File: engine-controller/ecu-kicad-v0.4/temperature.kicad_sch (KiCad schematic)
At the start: 70 parts, among them U31 AD8495, U32 TL431DBZ, U33 AD8495, U34 TL431DBZ, U35 AD8495, U36 AD8495, U37 TL431DBZ, U38 TL431DBZ, U39 AD8495, U40 TL431DBZ, U41 AD8495, U42 AD8495, U43 AD8495, U44 AD8495, U45 AD8495, U46 TL431DBZ, U47 TL431DBZ, U48 TL431DBZ, U49 TL431DBZ, U50 TL431DBZ

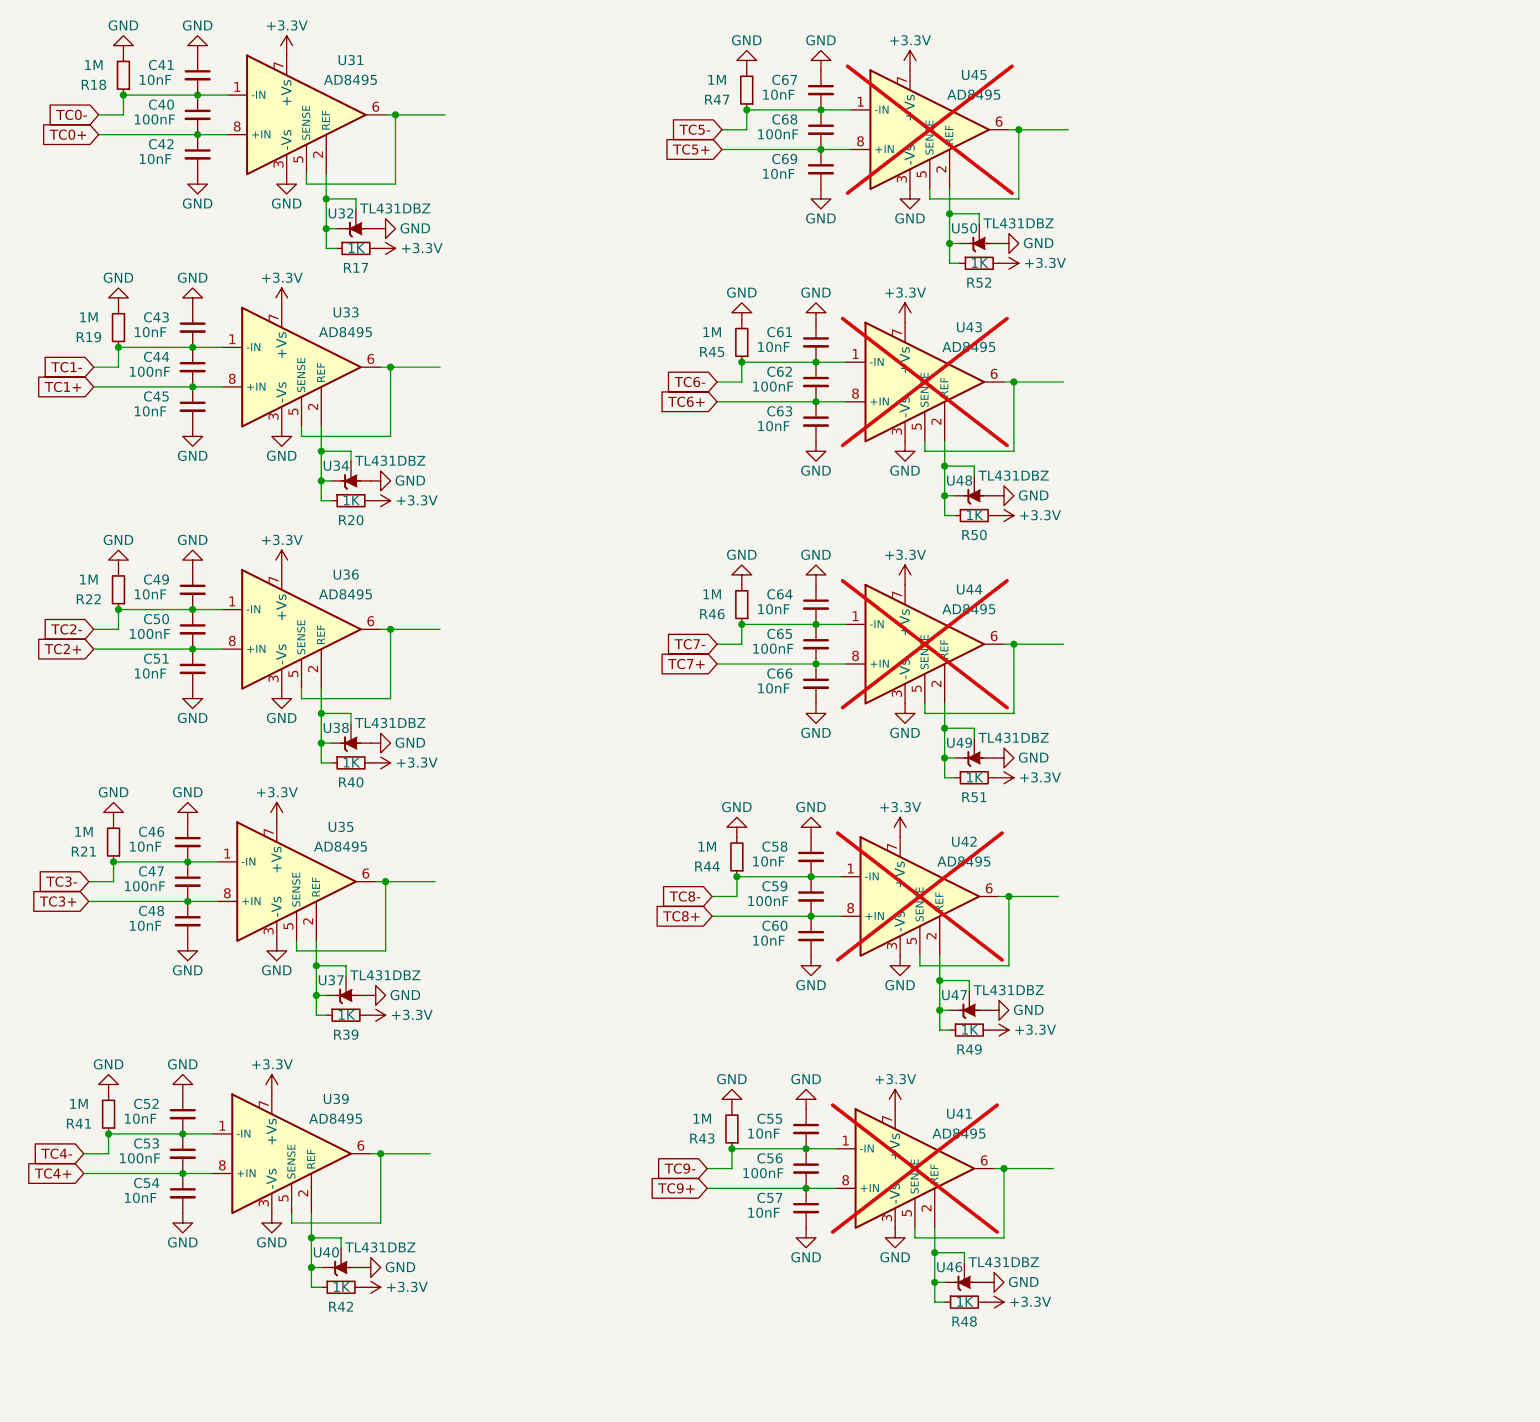
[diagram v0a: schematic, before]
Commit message: That's a lot of changes
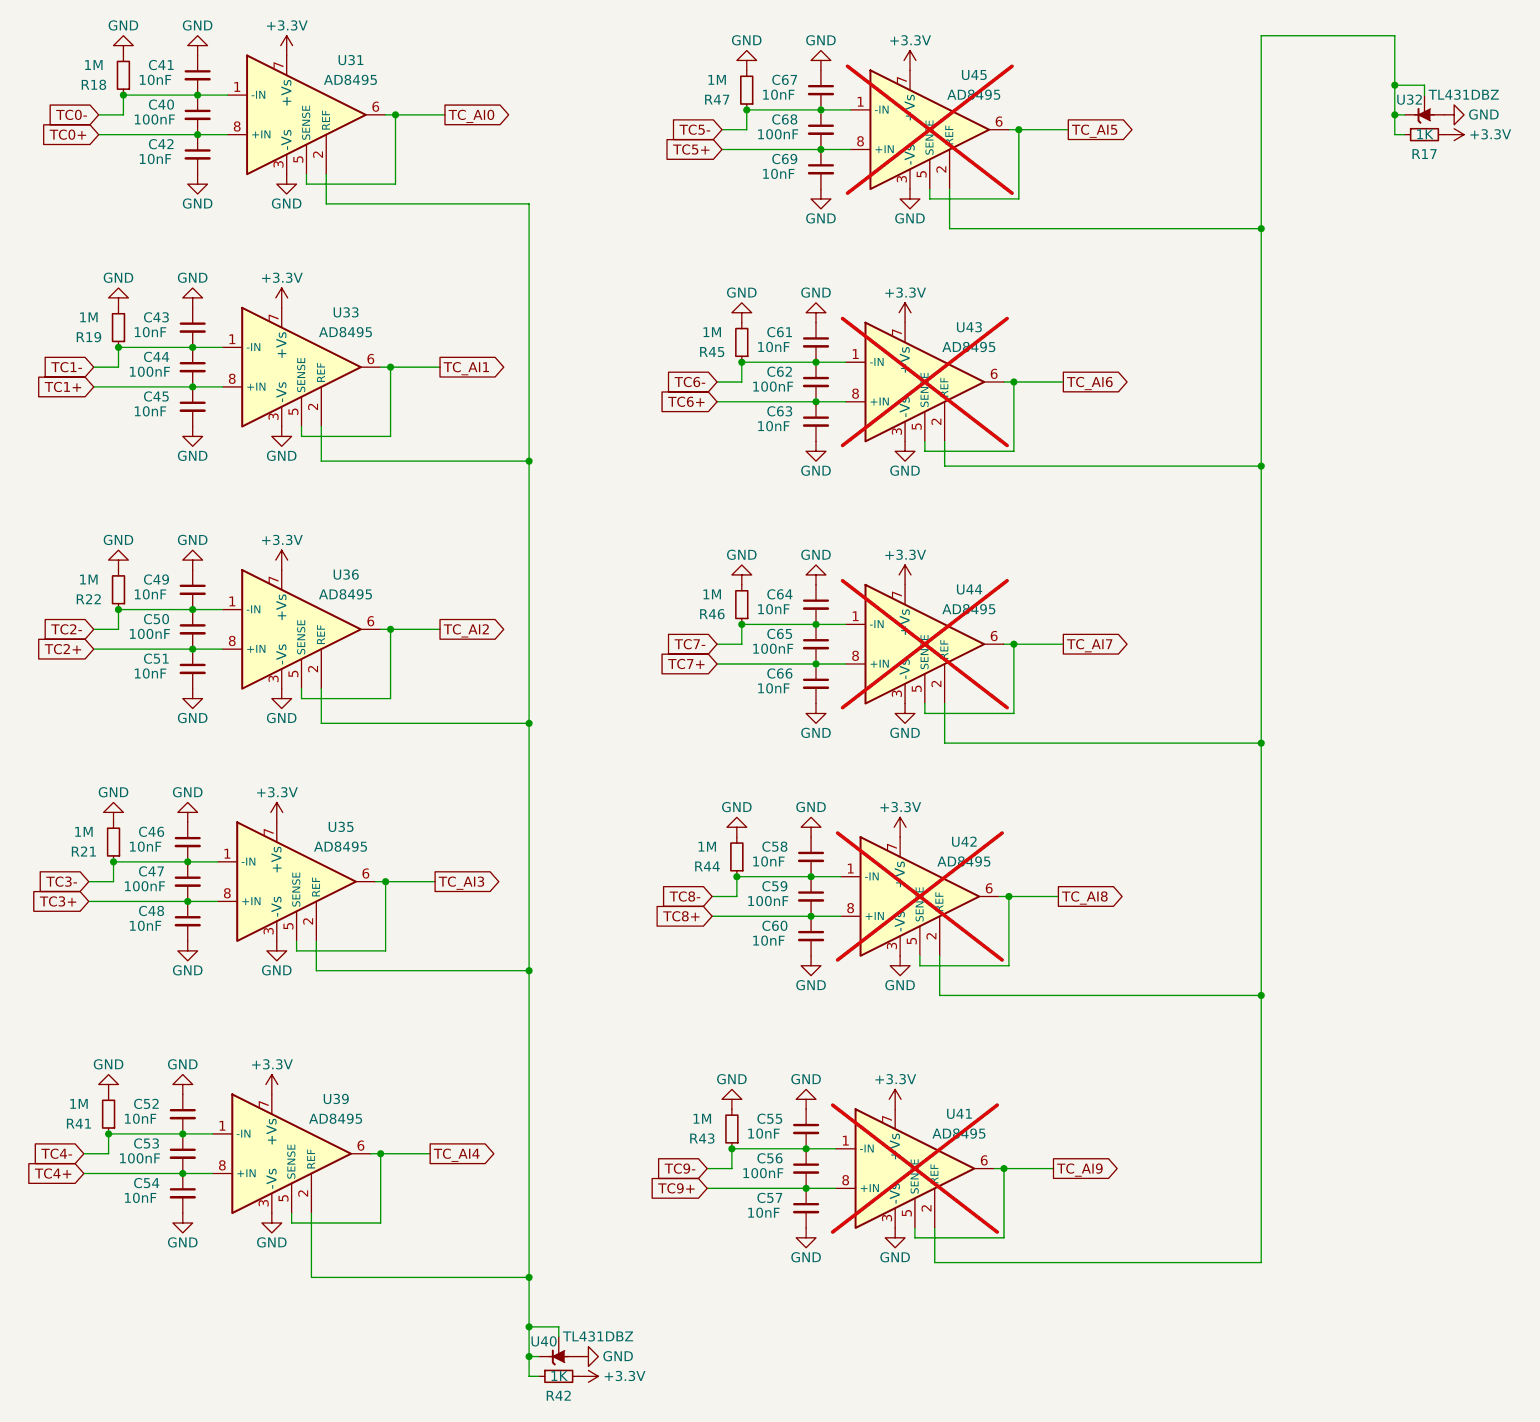
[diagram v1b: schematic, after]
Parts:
- removed R20, R39, R40, R48, R49, R50, R51, R52: 1K, Resistor_SMD:R_0603_1608Metric_Pad0.98x0.95mm_HandSolder, symbol Device:R_Small
- removed U34, U37, U38, U46, U47, U48, U49, U50: TL431DBZ, Package_TO_SOT_SMD:SOT-23, symbol Reference_Voltage:TL431DBZ
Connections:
- net at U42.2 (REF): now also R17.1, U32.1 (K), U32.2 (REF), U41.2 (REF), U43.2 (REF), U44.2 (REF), U45.2 (REF)
- net TC_AI8: now reaches U42.5 (SENSE), U42.6
- net TC_AI6: now reaches U43.5 (SENSE), U43.6
- net at R42.1, U39.2 (REF), U40.1 (K)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: now also U31.2 (REF), U33.2 (REF), U35.2 (REF), U36.2 (REF)
- net TC_AI4: now reaches U39.5 (SENSE), U39.6
- net TC_AI0: now reaches U31.5 (SENSE), U31.6
- net TC_AI9: now reaches U41.5 (SENSE), U41.6
- net TC_AI3: now reaches U35.5 (SENSE), U35.6
- net TC_AI1: now reaches U33.5 (SENSE), U33.6
- net TC_AI5: now reaches U45.5 (SENSE), U45.6
- net TC_AI7: now reaches U44.5 (SENSE), U44.6
- net TC_AI2: now reaches U36.5 (SENSE), U36.6
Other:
- moved on the sheet: R42, U40
